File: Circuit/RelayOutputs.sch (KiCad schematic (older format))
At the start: 24 parts, among them K201 Meisei-m4-24h, K202 Meisei-m4-24h, K203 Meisei-m4-24h, K204 Meisei-m4-24h, K205 Meisei-m4-24h, K206 Meisei-m4-24h, Q201 Q_NPN_BCE, Q202 Q_NPN_BCE, Q203 Q_NPN_BCE, Q204 Q_NPN_BCE, Q205 Q_NPN_BCE, Q206 Q_NPN_BCE

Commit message: Continued PCB work, placement started. Report and presentation also started
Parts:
- D201, D202, D203, D204, D205, D206: footprint (none) -> Diodes_SMD:D_0805
- Q201, Q202, Q203, Q204, Q205, Q206: symbol Q_NPN_BCE -> Q_NPN_BCE-RESCUE-ControlCircuit
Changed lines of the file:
@@
 EESchema Schematic File Version 2
+LIBS:ControlCircuit-rescue
 LIBS:power
 LIBS:device
@@
 $EndComp
 $Comp
-L Q_NPN_BCE Q204
+L Q_NPN_BCE-RESCUE-ControlCircuit Q204
 U 1 1 58ADF9C4
 P 6400 2400
+AR Path="/58ADF9C4" Ref="Q204"  Part="1"
+AR Path="/58ADF524/58ADF9C4" Ref="Q204"  Part="1"
 F 0 "Q204" V 6350 2100 50  0000 L CNN
 F 1 "Q_NPN_BCE" V 6250 1850 50  0000 L CNN
@@
 F 0 "D204" H 7450 2200 50  0000 C CNN
 F 1 "D" H 7450 2000 50  0000 C CNN
-F 2 "" H 7450 2100 50  0001 C CNN
+F 2 "Diodes_SMD:D_0805" H 7450 2100 50  0001 C CNN
 F 3 "" H 7450 2100 50  0000 C CNN
 	1    7450 2100
@@
 $EndComp
 $Comp
-L Q_NPN_BCE Q205
+L Q_NPN_BCE-RESCUE-ControlCircuit Q205
 U 1 1 58AE896D
 P 6400 3800
+AR Path="/58AE896D" Ref="Q205"  Part="1"
+AR Path="/58ADF524/58AE896D" Ref="Q205"  Part="1"
 F 0 "Q205" V 6350 3500 50  0000 L CNN
 F 1 "Q_NPN_BCE" V 6250 3250 50  0000 L CNN
@@
 F 0 "D205" H 7450 3600 50  0000 C CNN
 F 1 "D" H 7450 3400 50  0000 C CNN
-F 2 "" H 7450 3500 50  0001 C CNN
+F 2 "Diodes_SMD:D_0805" H 7450 3500 50  0001 C CNN
 F 3 "" H 7450 3500 50  0000 C CNN
 	1    7450 3500
@@
 $EndComp
 $Comp
-L Q_NPN_BCE Q206
+L Q_NPN_BCE-RESCUE-ControlCircuit Q206
 U 1 1 58AE8A45
 P 6400 5200
+AR Path="/58AE8A45" Ref="Q206"  Part="1"
+AR Path="/58ADF524/58AE8A45" Ref="Q206"  Part="1"
 F 0 "Q206" V 6350 4900 50  0000 L CNN
 F 1 "Q_NPN_BCE" V 6250 4650 50  0000 L CNN
@@
 F 0 "D206" H 7450 5000 50  0000 C CNN
 F 1 "D" H 7450 4800 50  0000 C CNN
-F 2 "" H 7450 4900 50  0001 C CNN
+F 2 "Diodes_SMD:D_0805" H 7450 4900 50  0001 C CNN
 F 3 "" H 7450 4900 50  0000 C CNN
 	1    7450 4900
@@
 $EndComp
 $Comp
-L Q_NPN_BCE Q201
+L Q_NPN_BCE-RESCUE-ControlCircuit Q201
 U 1 1 58AE8E1D
 P 3500 2350
+AR Path="/58AE8E1D" Ref="Q201"  Part="1"
+AR Path="/58ADF524/58AE8E1D" Ref="Q201"  Part="1"
 F 0 "Q201" V 3450 2050 50  0000 L CNN
 F 1 "Q_NPN_BCE" V 3350 1800 50  0000 L CNN
@@
 F 0 "D201" H 4550 2150 50  0000 C CNN
 F 1 "D" H 4550 1950 50  0000 C CNN
-F 2 "" H 4550 2050 50  0001 C CNN
+F 2 "Diodes_SMD:D_0805" H 4550 2050 50  0001 C CNN
 F 3 "" H 4550 2050 50  0000 C CNN
 	1    4550 2050
@@
 $EndComp
 $Comp
-L Q_NPN_BCE Q202
+L Q_NPN_BCE-RESCUE-ControlCircuit Q202
 U 1 1 58AE8E5D
 P 3500 3750
+AR Path="/58AE8E5D" Ref="Q202"  Part="1"
+AR Path="/58ADF524/58AE8E5D" Ref="Q202"  Part="1"
 F 0 "Q202" V 3450 3450 50  0000 L CNN
 F 1 "Q_NPN_BCE" V 3350 3200 50  0000 L CNN
@@
 F 0 "D202" H 4550 3550 50  0000 C CNN
 F 1 "D" H 4550 3350 50  0000 C CNN
-F 2 "" H 4550 3450 50  0001 C CNN
+F 2 "Diodes_SMD:D_0805" H 4550 3450 50  0001 C CNN
 F 3 "" H 4550 3450 50  0000 C CNN
 	1    4550 3450
@@
 $EndComp
 $Comp
-L Q_NPN_BCE Q203
+L Q_NPN_BCE-RESCUE-ControlCircuit Q203
 U 1 1 58AE8E9D
 P 3500 5150
+AR Path="/58AE8E9D" Ref="Q203"  Part="1"
+AR Path="/58ADF524/58AE8E9D" Ref="Q203"  Part="1"
 F 0 "Q203" V 3450 4850 50  0000 L CNN
 F 1 "Q_NPN_BCE" V 3350 4600 50  0000 L CNN
@@
 F 0 "D203" H 4550 4950 50  0000 C CNN
 F 1 "D" H 4550 4750 50  0000 C CNN
-F 2 "" H 4550 4850 50  0001 C CNN
+F 2 "Diodes_SMD:D_0805" H 4550 4850 50  0001 C CNN
 F 3 "" H 4550 4850 50  0000 C CNN
 	1    4550 4850

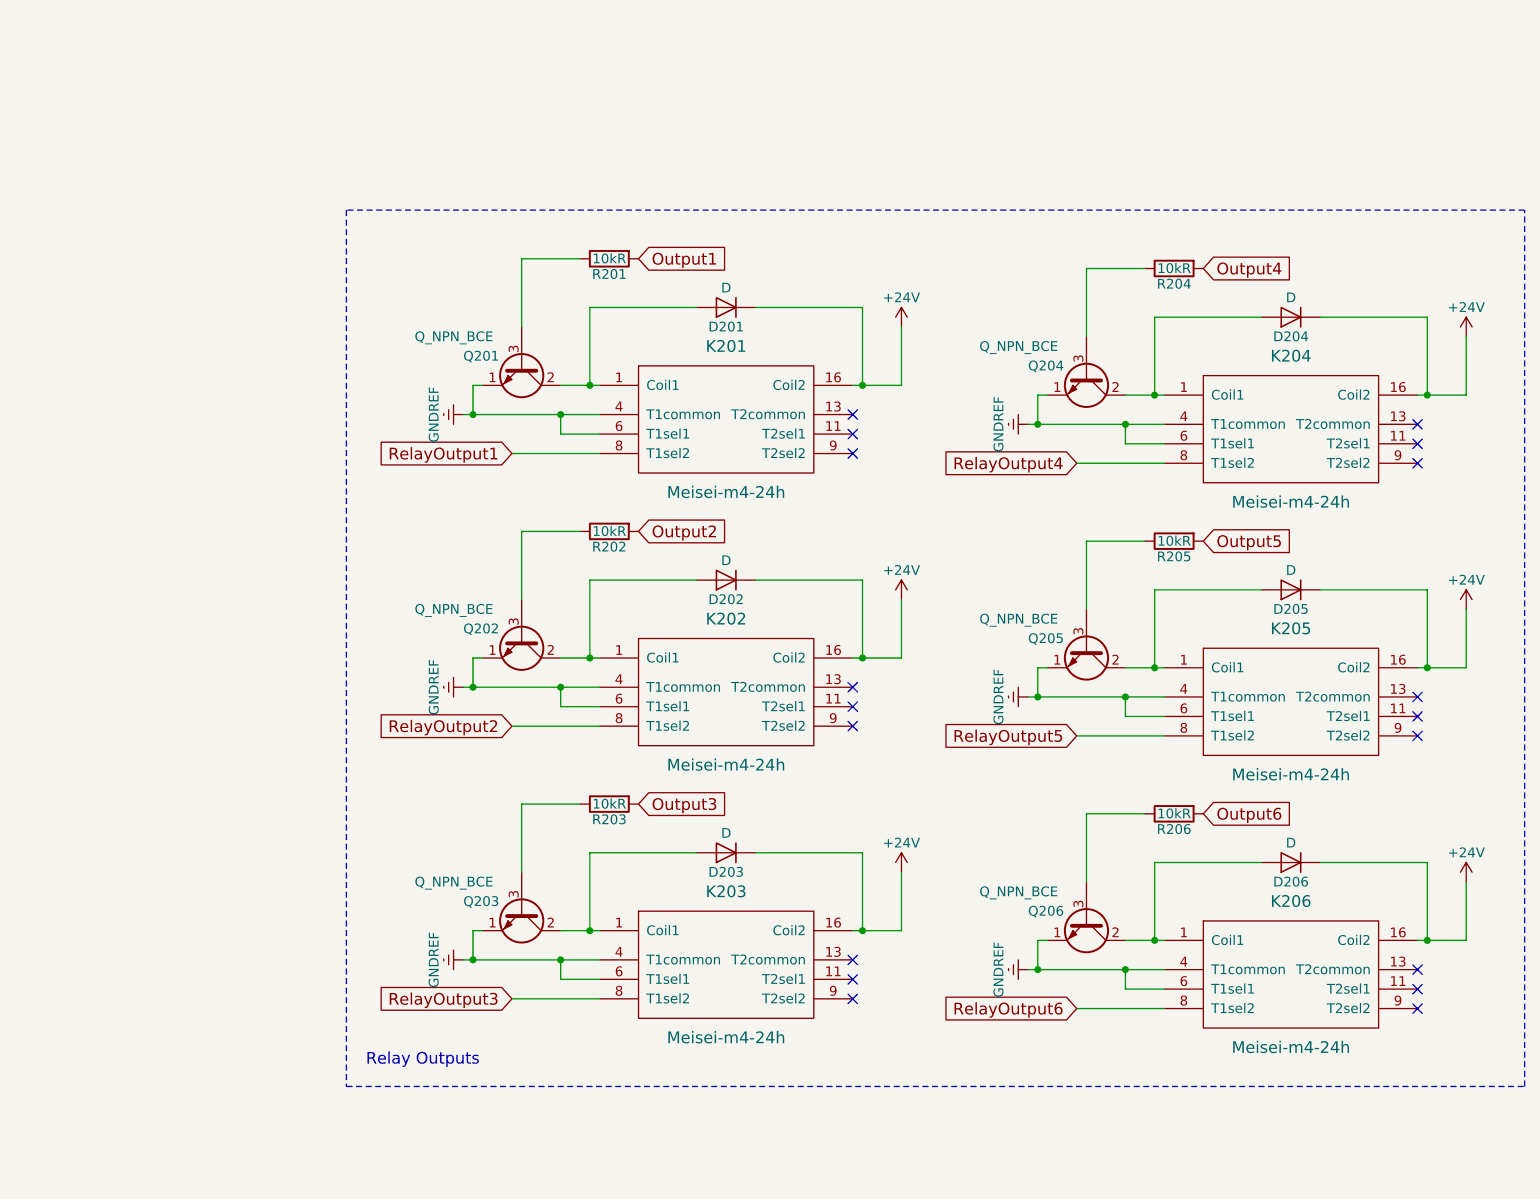
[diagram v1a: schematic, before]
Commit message: Continued PCB work, additional footprints added
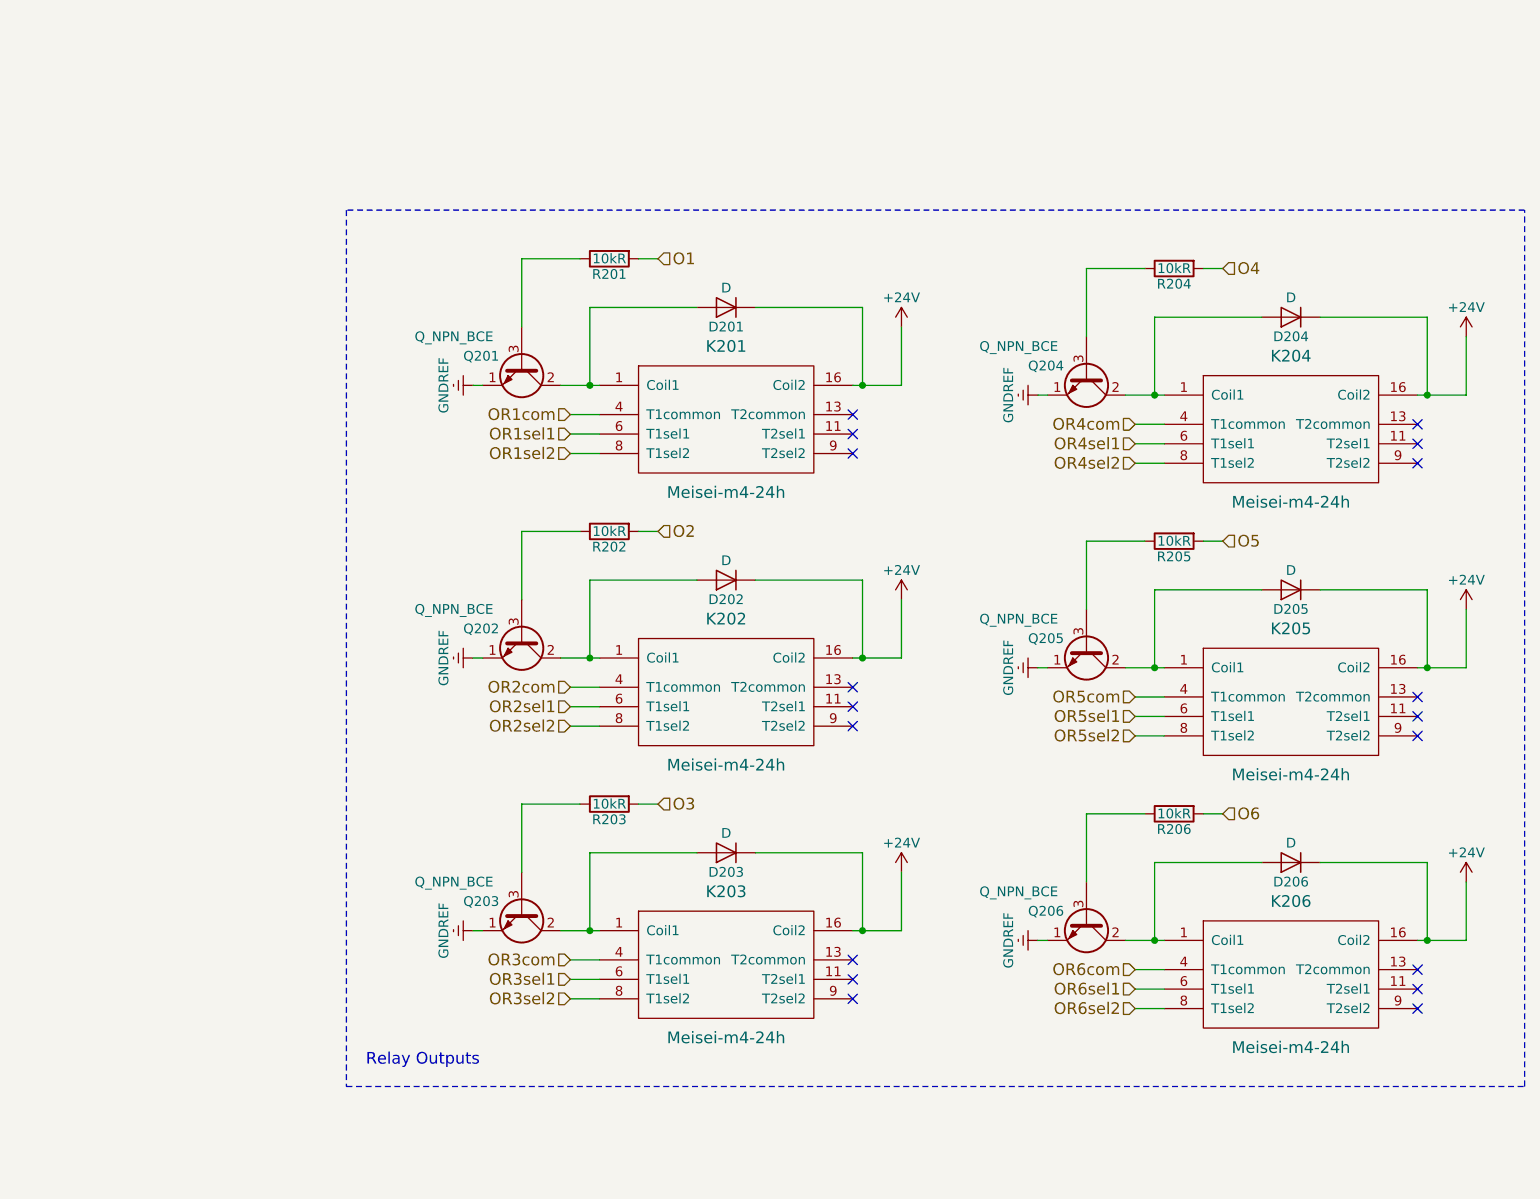
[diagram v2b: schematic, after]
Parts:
- D201, D202, D203, D204, D205, D206: footprint Diodes_SMD:D_0805 -> Diodes_SMD:D_MiniMELF_Standard
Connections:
- net GNDREF: no longer K201.4 (T1common), K201.6 (T1sel1), K202.4 (T1common), K202.6 (T1sel1), K203.4 (T1common), K203.6 (T1sel1), K204.4 (T1common), K204.6 (T1sel1), K205.4 (T1common), K205.6 (T1sel1), K206.4 (T1common), K206.6 (T1sel1)
- net Output1 renamed O1
- net Output2 renamed O2
- net Output3 renamed O3
- net Output4 renamed O4
- net Output5 renamed O5
- net Output6 renamed O6
- net RelayOutput1 renamed OR1sel2
- net RelayOutput2 renamed OR2sel2
- net RelayOutput3 renamed OR3sel2
- net RelayOutput4 renamed OR4sel2
- net RelayOutput5 renamed OR5sel2
- net RelayOutput6 renamed OR6sel2
- new net OR1com: K201.4 (T1common)
- new net OR1sel1: K201.6 (T1sel1)
- new net OR2com: K202.4 (T1common)
- new net OR2sel1: K202.6 (T1sel1)
- new net OR3com: K203.4 (T1common)
- new net OR3sel1: K203.6 (T1sel1)
- new net OR4com: K204.4 (T1common)
- new net OR4sel1: K204.6 (T1sel1)
- new net OR5com: K205.4 (T1common)
- new net OR5sel1: K205.6 (T1sel1)
- new net OR6com: K206.4 (T1common)
- new net OR6sel1: K206.6 (T1sel1)

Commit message: Additional PCB work
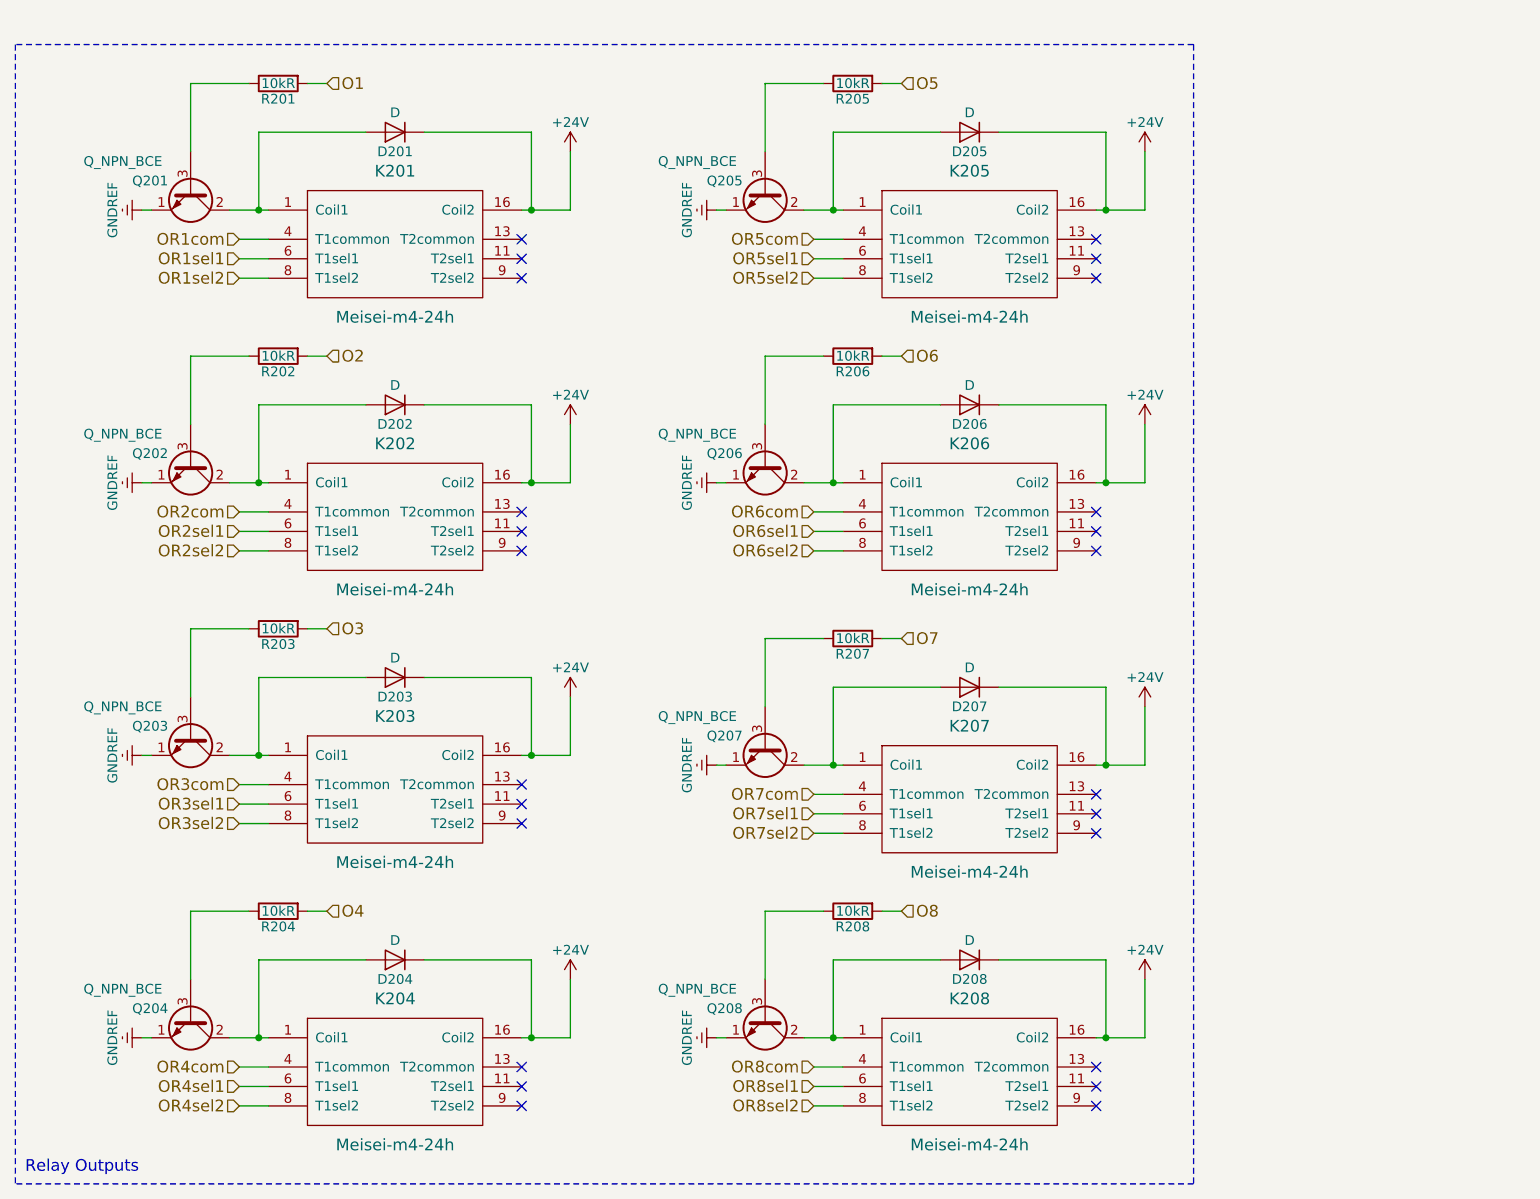
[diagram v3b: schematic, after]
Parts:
- added D207, D208: D, Diodes_SMD:D_MiniMELF_Standard, symbol D
- added K207, K208: Meisei-m4-24h, Meisei:Meisei-m4-24h, symbol Meisei-m4-24h
- added Q207, Q208: Q_NPN_BCE, MMBT3904:MMBT3904, symbol Q_NPN_BCE-RESCUE-ControlCircuit
- added R207, R208: 10kR, Resistors_SMD:R_0805, symbol R
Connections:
- net +24V: now also D207.1 (K), D208.1 (K), K207.16 (Coil2), K208.16 (Coil2)
- net GNDREF: now also Q207.1 (E), Q208.1 (E)
- new net: D207.2 (A), K207.1 (Coil1), Q207.2 (C)
- new net: Q207.3 (B), R207.1
- new net: D208.2 (A), K208.1 (Coil1), Q208.2 (C)
- new net: Q208.3 (B), R208.1
- new net O7: R207.2
- new net O8: R208.2
- new net OR7com: K207.4 (T1common)
- new net OR7sel1: K207.6 (T1sel1)
- new net OR7sel2: K207.8 (T1sel2)
- new net OR8com: K208.4 (T1common)
- new net OR8sel1: K208.6 (T1sel1)
- new net OR8sel2: K208.8 (T1sel2)
- no-connect marks 18 -> 24
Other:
- moved on the sheet: D201, D202, D203, D204, D205, D206, K201, K202, K203, K204, K205, K206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
